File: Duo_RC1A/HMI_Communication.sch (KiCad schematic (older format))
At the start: 29 parts, among them P1 HEADER_180_2.54_10X2, P2 KK3.96_2, U1 SN75176BDR

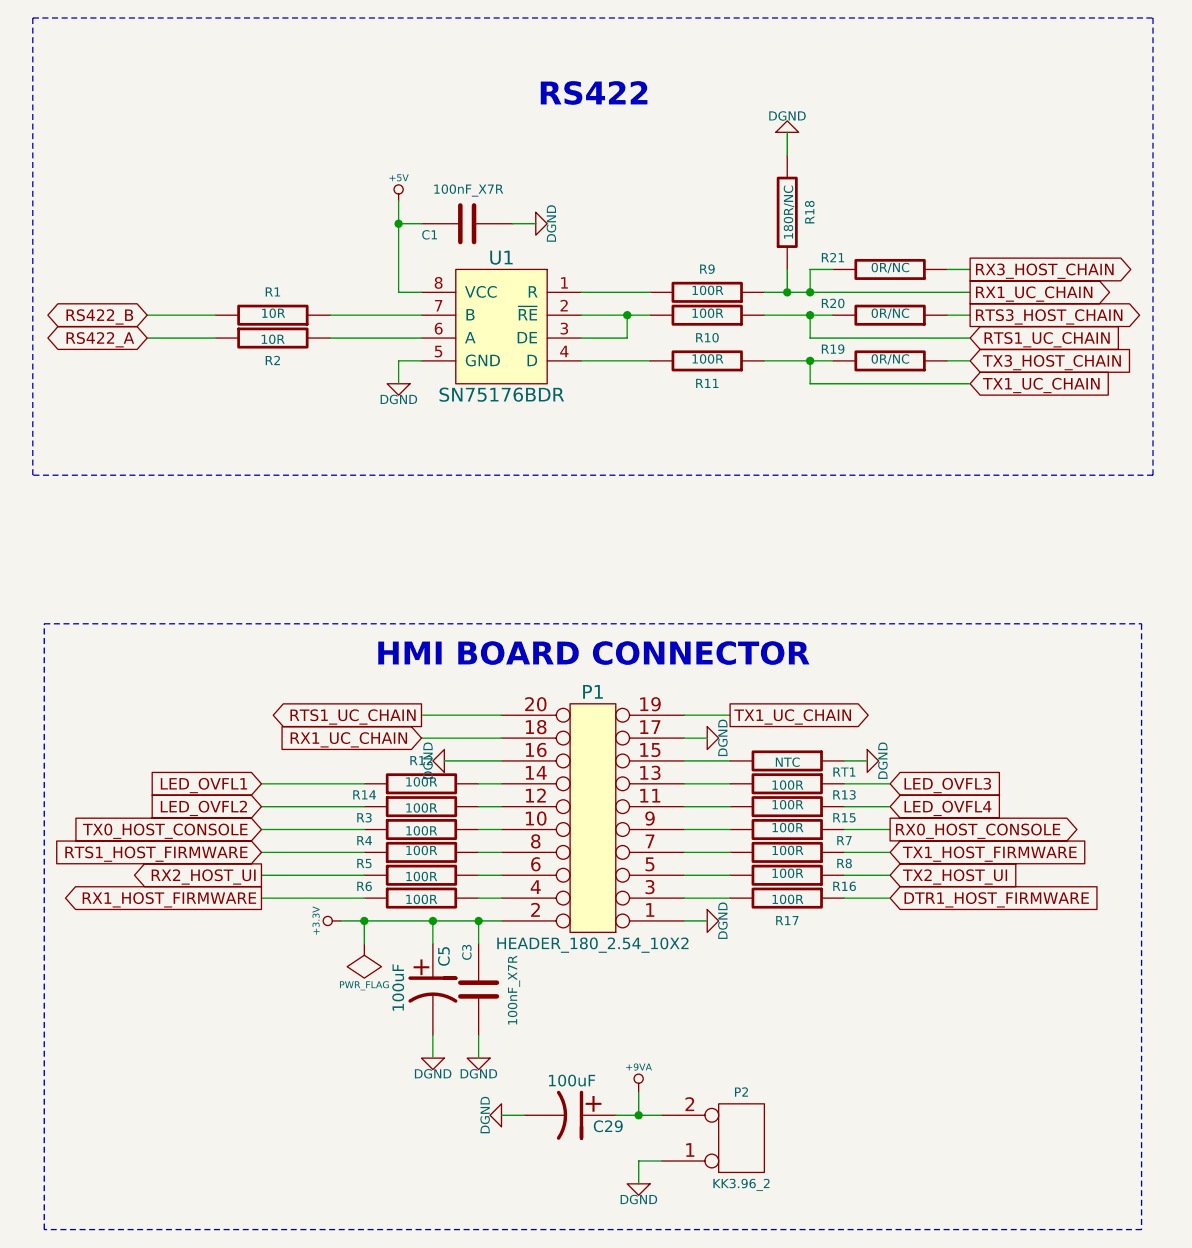
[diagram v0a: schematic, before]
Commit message: Wrking on the sound. Changed the board size.
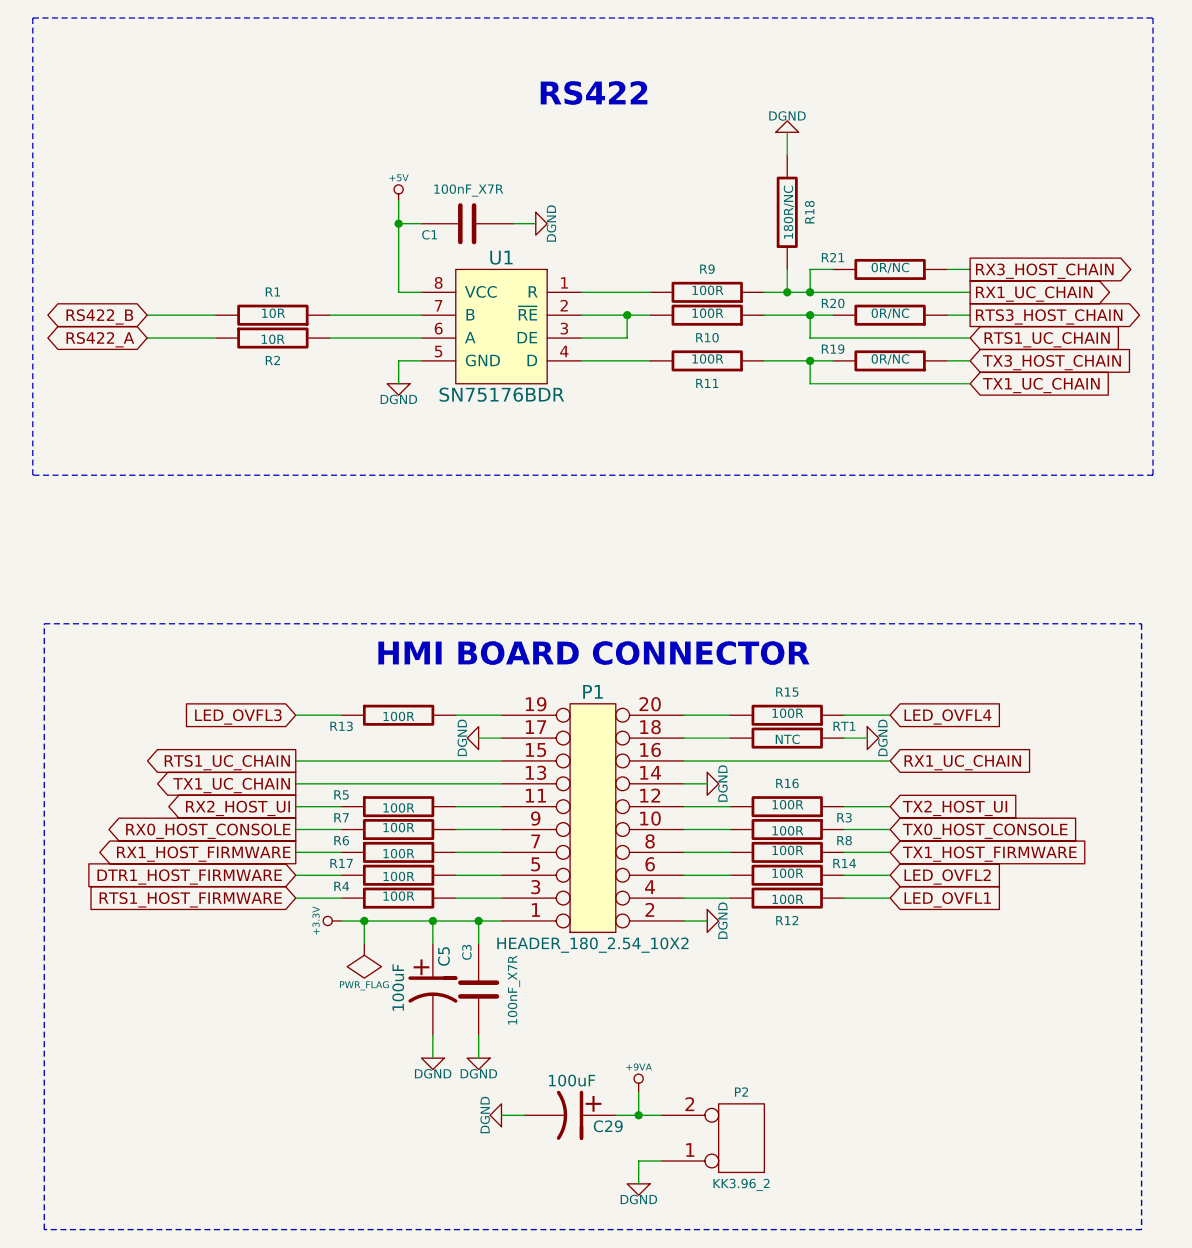
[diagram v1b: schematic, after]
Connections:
- net +3.3V: now also P1.1 (P1); no longer P1.2 (P2)
- net DGND: now also P1.14 (P14), P1.2 (P2); no longer P1.1 (P1), P1.16 (P16)
- net RTS1_UC_CHAIN: now also P1.15 (P15); no longer P1.20 (P20)
- net RX1_UC_CHAIN: now also P1.16 (P16); no longer P1.18 (P18)
- net TX1_UC_CHAIN: now also P1.13 (P13); no longer P1.19 (P19)
- net at P1.11 (P11): now also R5.2; no longer R15.2
- net at P1.12 (P12): now also R16.2; no longer R14.2
- net at R13.2: now also P1.19 (P19); no longer P1.13 (P13)
- net at R12.2: now also P1.4 (P4); no longer P1.14 (P14)
- net at RT1.2: now also P1.18 (P18); no longer P1.15 (P15)
- net at P1.3 (P3): now also R4.2; no longer R17.2
- net at R6.2: now also P1.7 (P7); no longer P1.4 (P4)
- net at P1.5 (P5): now also R17.2; no longer R16.2
- net at P1.6 (P6): now also R14.2; no longer R5.2
- net at R8.2: now also P1.8 (P8); no longer P1.7 (P7)
- new net: P1.20 (P20), R15.2
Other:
- moved on the sheet: R12, R13, R14, R15, R16, R17, R3, R4, R5, R6, R7, RT1
